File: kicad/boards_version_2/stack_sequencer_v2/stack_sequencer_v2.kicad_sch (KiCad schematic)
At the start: 14 parts

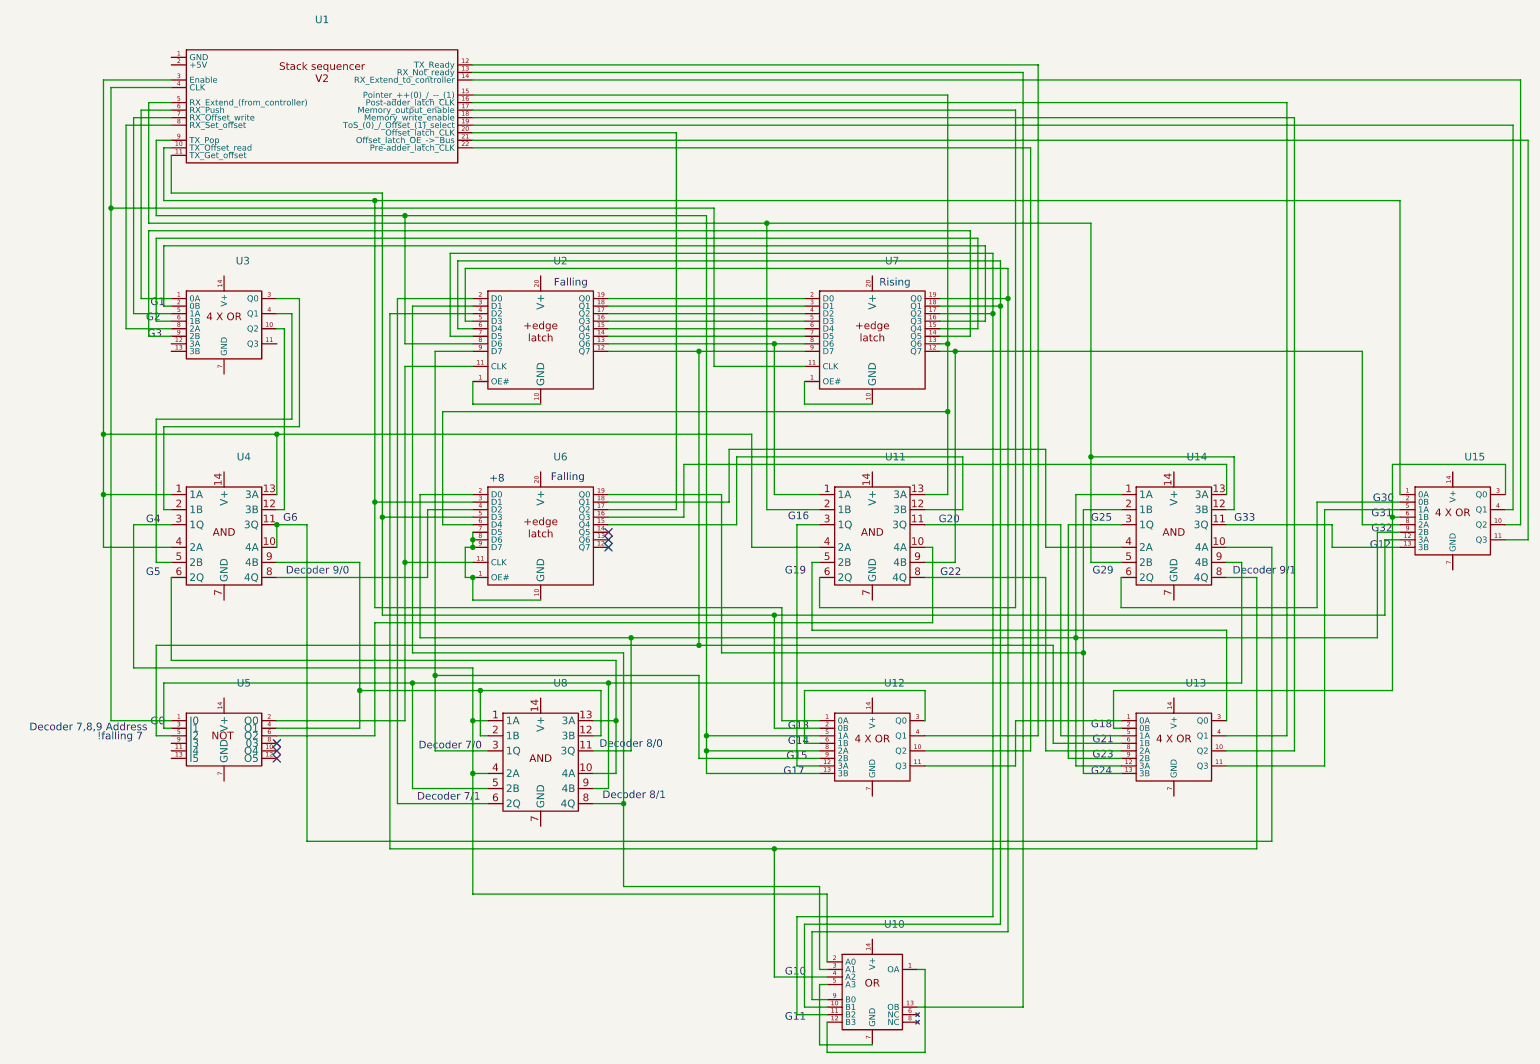
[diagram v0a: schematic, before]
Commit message: Stack sequencer verified
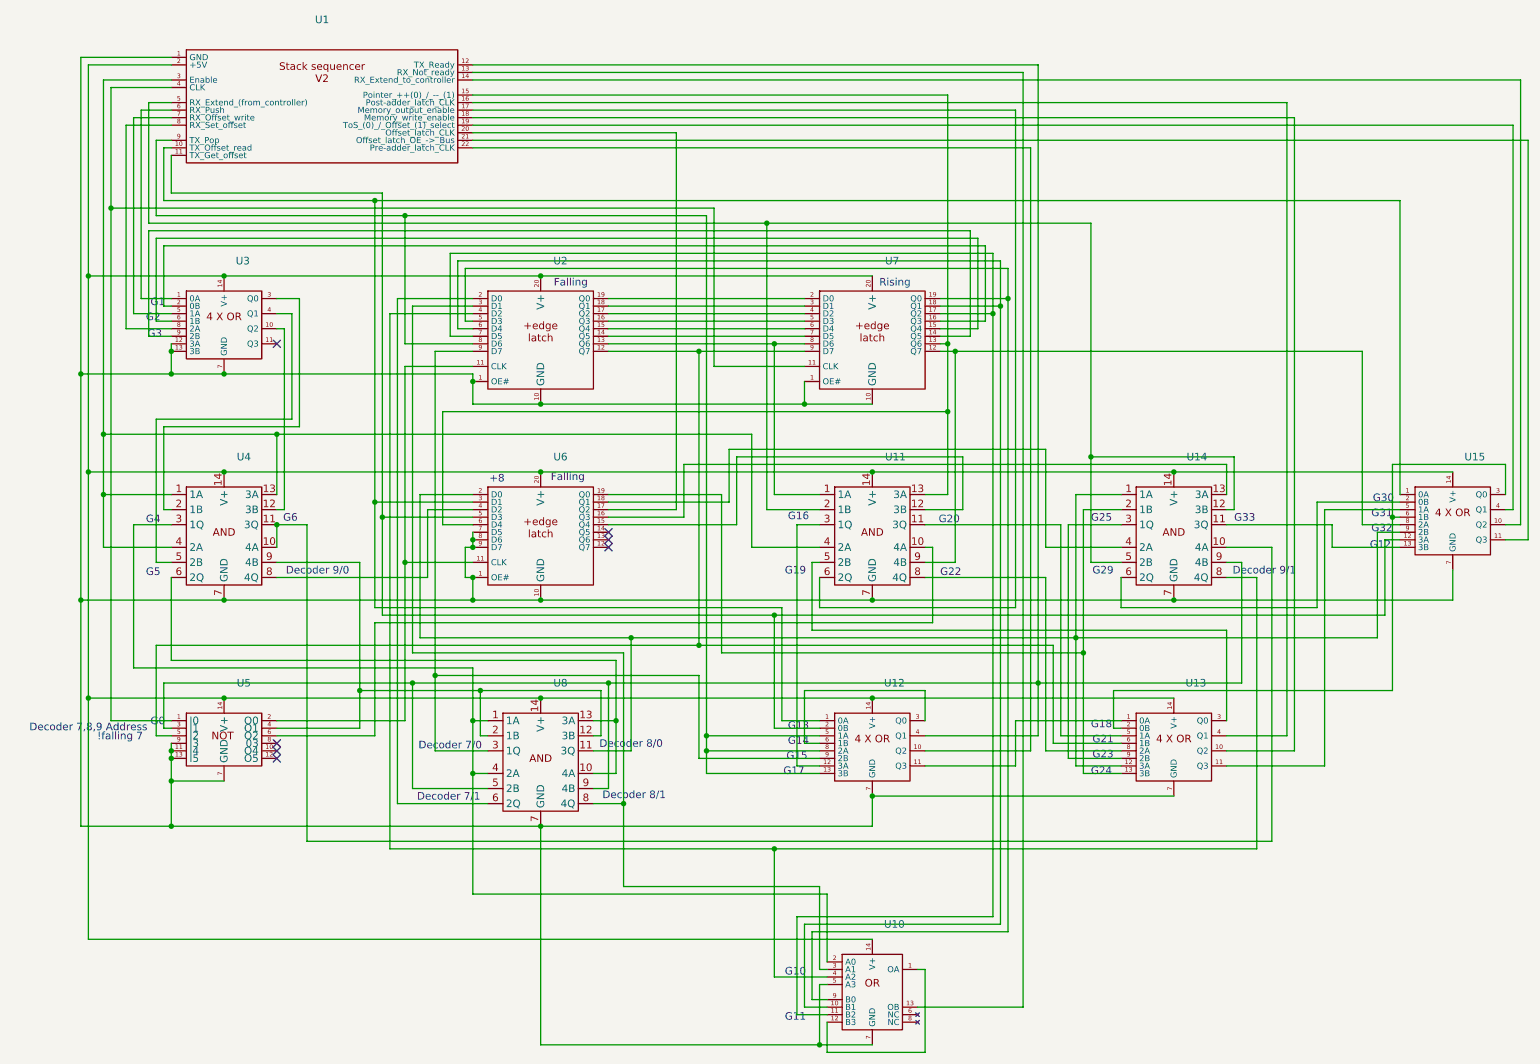
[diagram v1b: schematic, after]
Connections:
- net at U3.12 (3A): now also U1.1 (GND), U10.5 (A3), U10.7 (GND), U11.7 (GND), U12.7 (GND), U13.7 (GND), U14.7 (GND), U15.7 (GND), U2.1 (OE#), U2.10 (GND), U3.13 (3B), U3.7 (GND), U4.7 (GND), U5.11 (I4), U5.13 (I5), U5.7 (GND), U5.9 (I3), U6.1 (OE#), U6.10 (GND), U6.7 (D5), U6.8 (D6), U6.9 (D7), U7.1 (OE#), U7.10 (GND), U8.7 (GND)
- net at U3.14 (V+): now also U1.2 (+5V), U10.14 (V+), U11.14 (V+), U12.14 (V+), U13.14 (V+), U14.14 (V+), U15.14 (V+), U2.20 (V+), U4.14 (V+), U5.14 (V+), U6.20 (V+), U7.20 (V+), U8.14 (V+)
- net at U14.9 (4B), U5.3 (I1), U8.5 (2B)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: now also U1.12 (TX_Ready), U12.4 (Q1)
- no-connect marks 6 -> 7
